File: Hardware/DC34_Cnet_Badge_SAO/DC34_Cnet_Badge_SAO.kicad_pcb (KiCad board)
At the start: 2 copper layers, 49.8 x 49.9 mm, 4 parts, among them J1 Conn_02x03_Top_Bottom

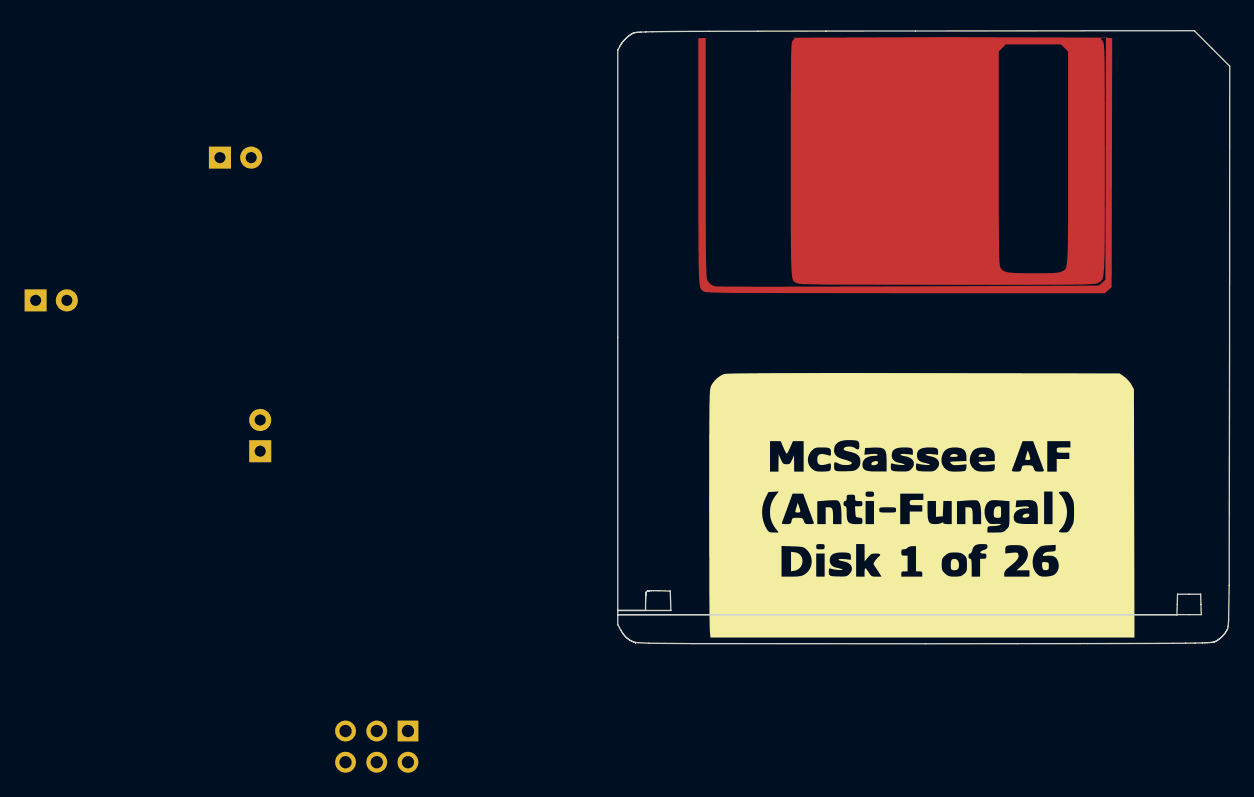
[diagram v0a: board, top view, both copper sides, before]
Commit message: Updates
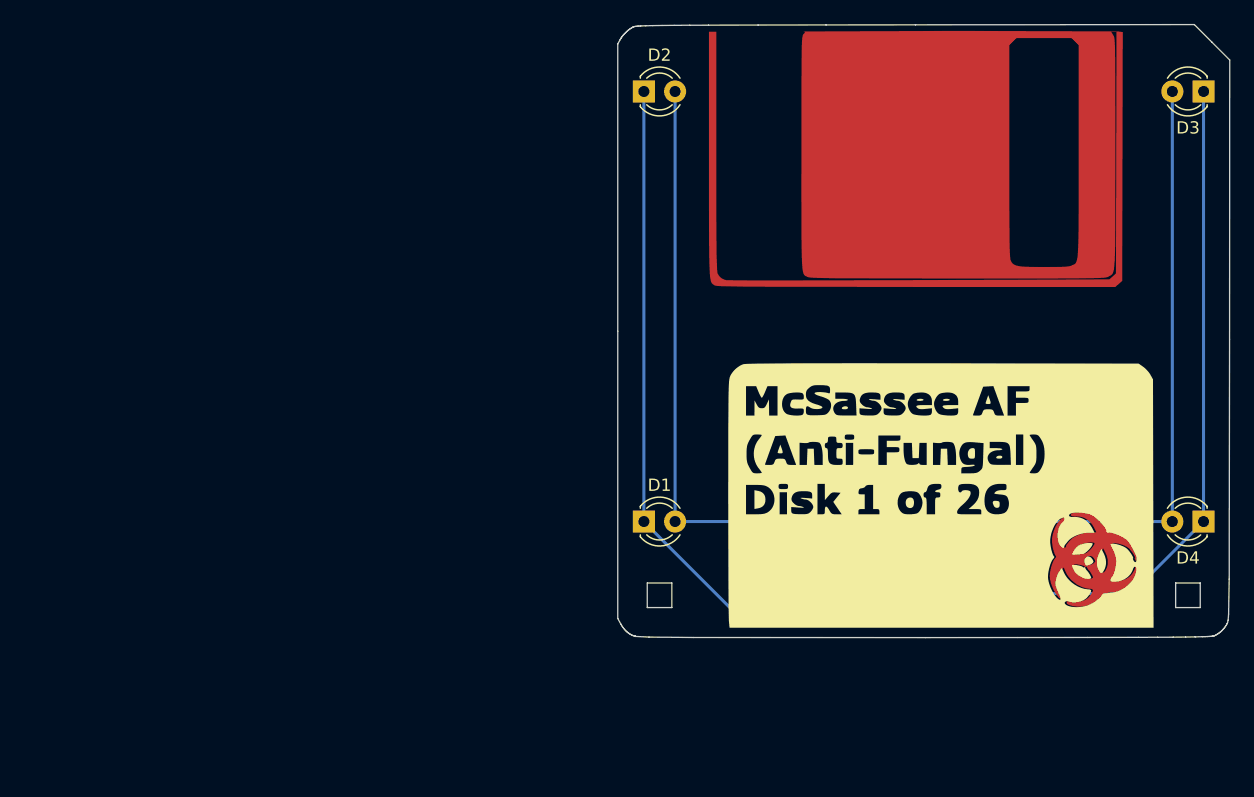
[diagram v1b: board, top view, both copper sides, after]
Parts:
- added D4: LED, LED_THT:LED_D3.0mm, F.Cu at (169.3, 120.0)
- D1, D2, D3: moved to F.Cu
- moved D3 80.2 mm to (169.3, 85.0), turned to 180 degrees
- moved D2 52.3 mm to (123.7, 85.0)
- moved J1 46.7 mm to (149.5, 124.5)
- moved D1 31.7 mm to (123.7, 120.0), turned to 0 degrees
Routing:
- net GND: track 0.00 -> 121.4 mm
- net +3.3V: track 0.00 -> 114.2 mm
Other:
- outline, holes or cut-outs redrawn

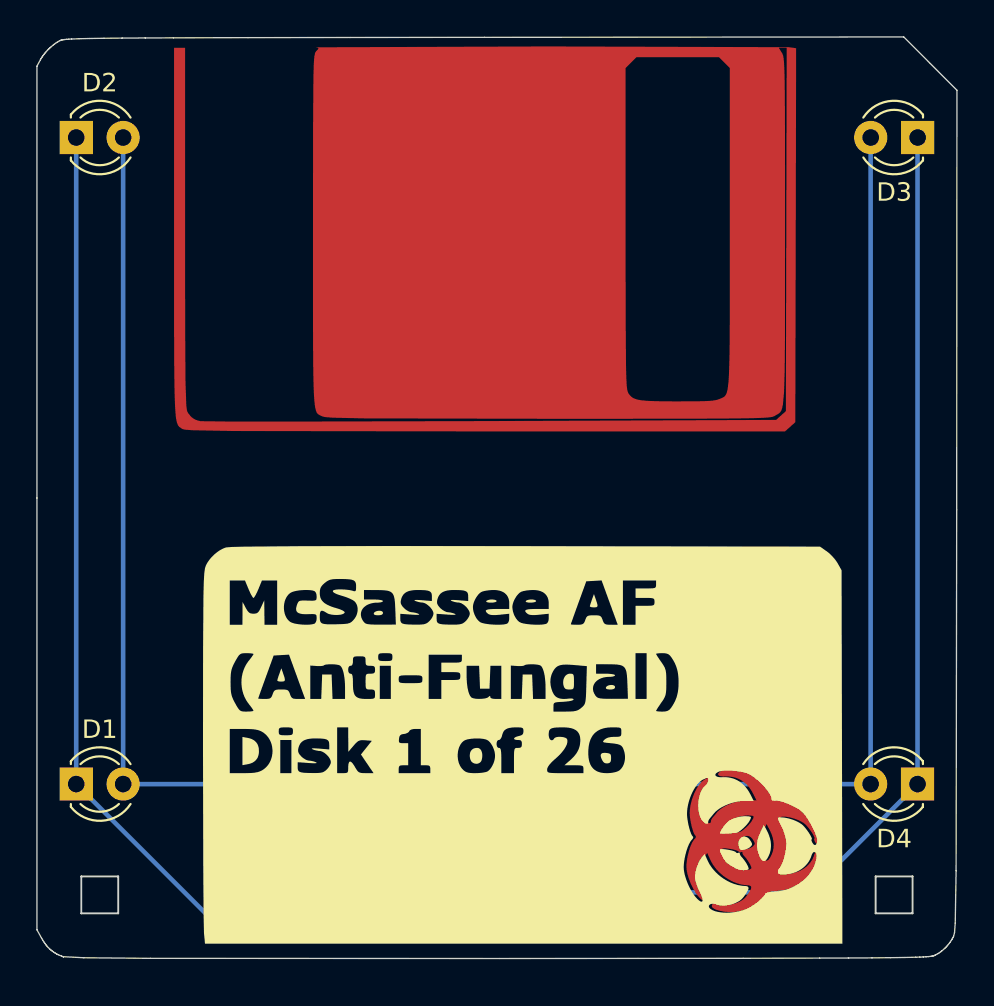
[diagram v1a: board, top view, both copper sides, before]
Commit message: PCB Updates
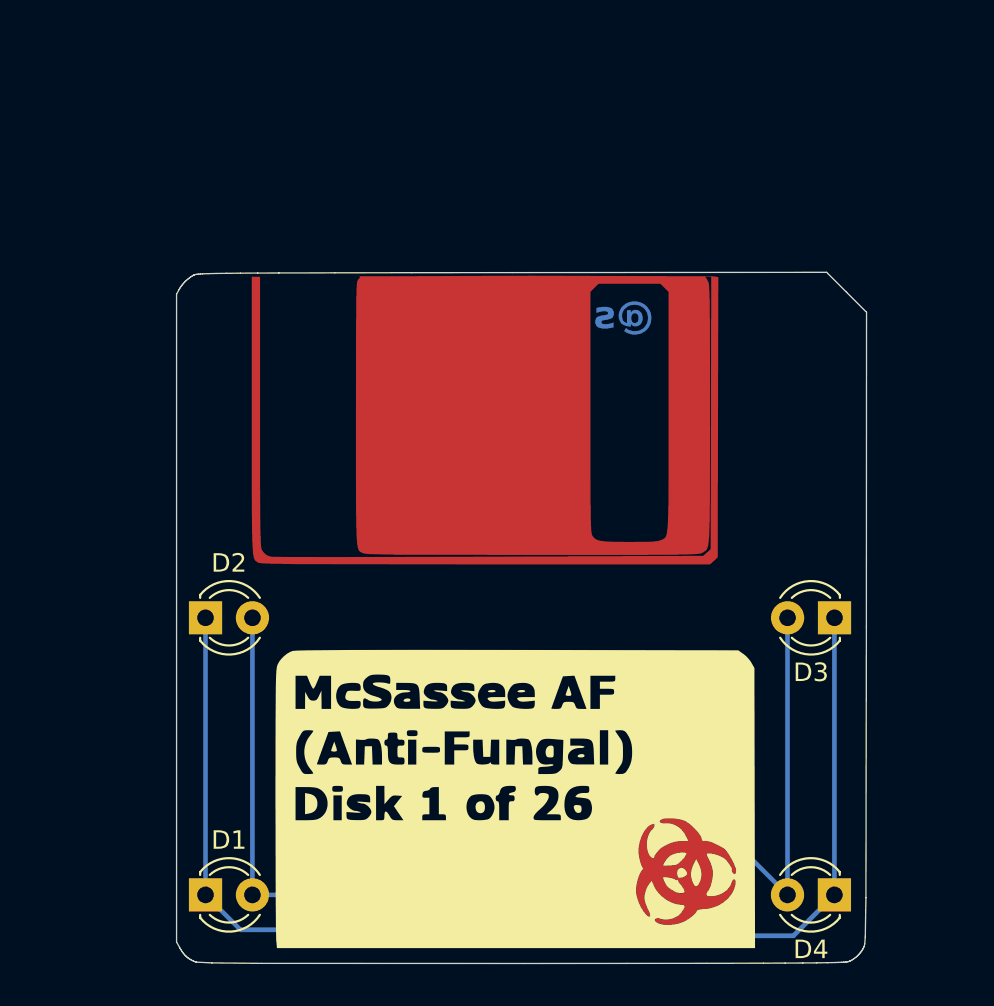
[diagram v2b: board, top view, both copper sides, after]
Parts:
- moved D2 26.9 mm to (130.7, 111.0)
- moved D3 26.4 mm to (164.8, 111.0)
- moved D1 9.22 mm to (130.7, 126.0)
- moved D4 7.50 mm to (164.8, 126.0)
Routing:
- net GND: track 121.4 -> 66.6 mm
- net +3.3V: track 114.2 -> 61.2 mm
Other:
- board size 49.8 x 49.9 mm -> 37.4 x 37.4 mm
- board text added: "@slash128v6"
